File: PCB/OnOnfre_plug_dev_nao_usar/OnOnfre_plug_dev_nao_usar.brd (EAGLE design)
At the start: 44.4 x 47.7 mm, 41 parts, among them IC4 HLW8012, J7 8p, Q3 2N7002, Q4 2N7002, U2 esp12

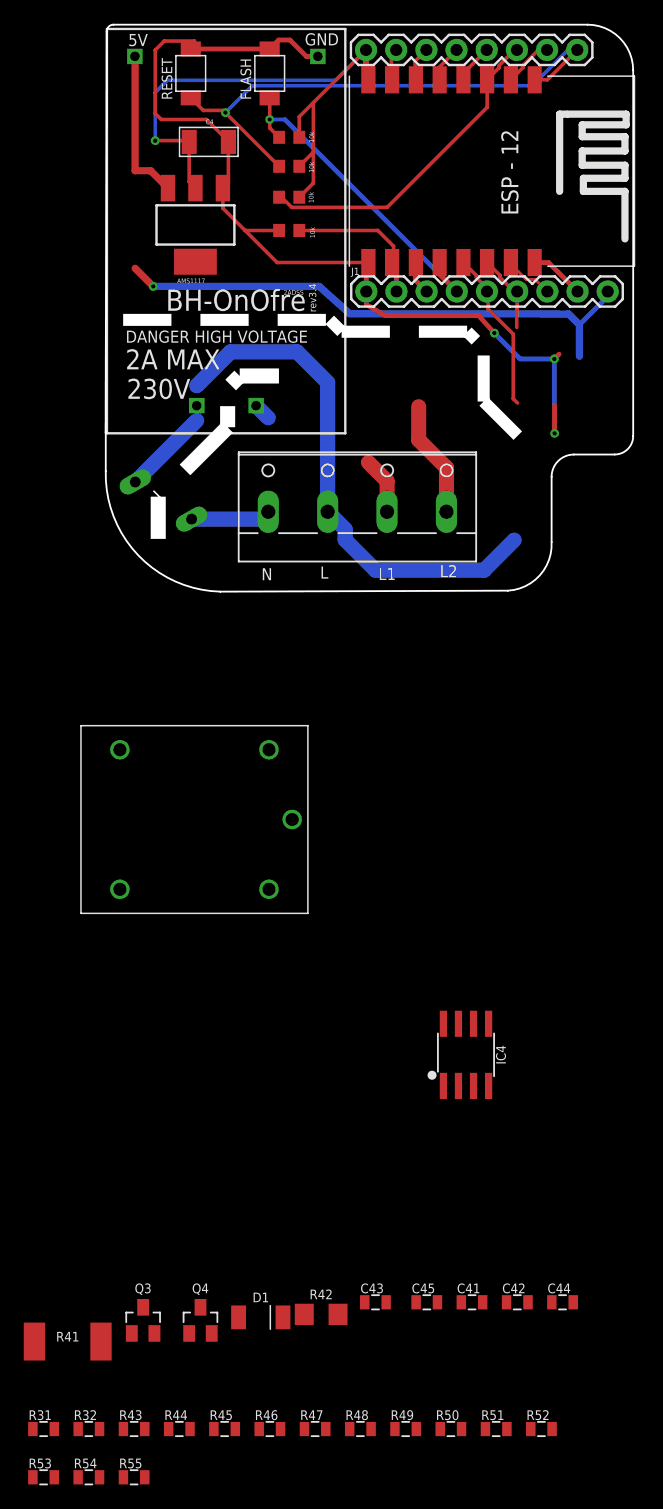
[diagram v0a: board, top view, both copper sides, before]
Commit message: Labels Fix
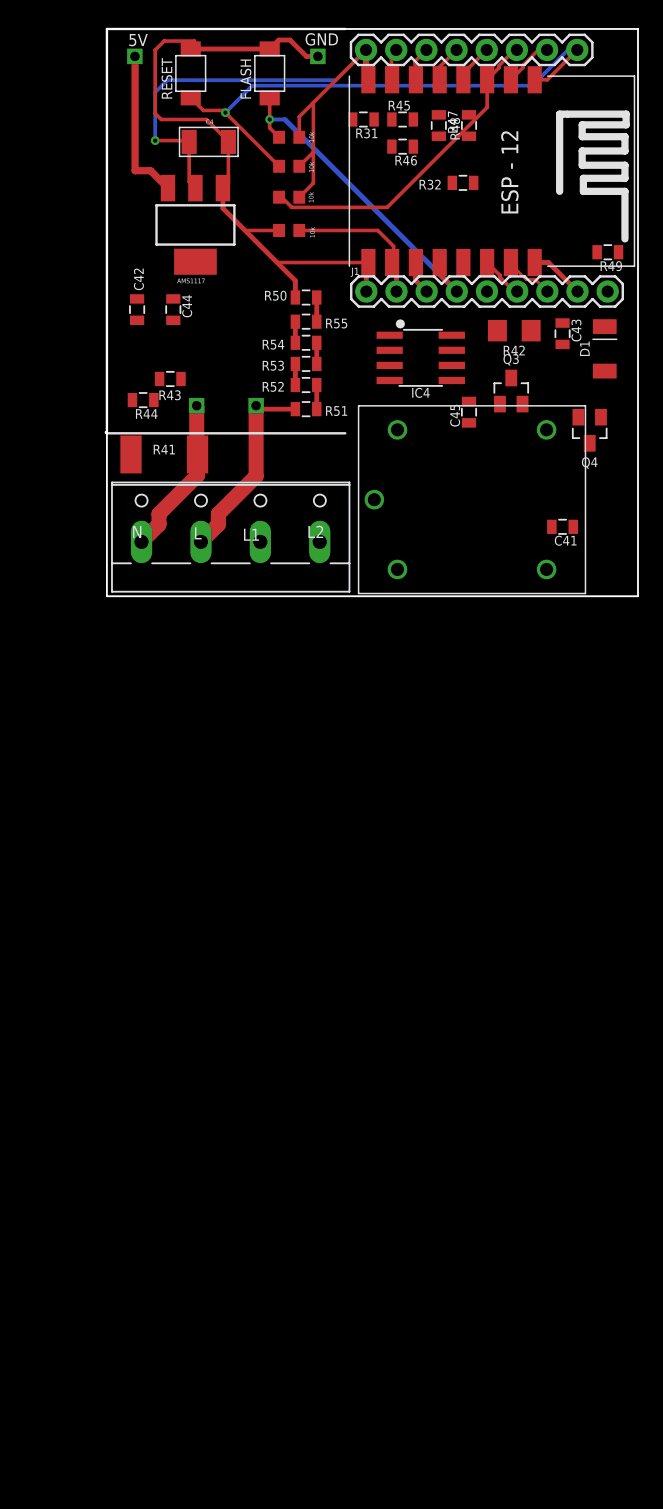
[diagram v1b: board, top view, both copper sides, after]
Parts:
- removed R5: VARISTORS07K230, varistor:S07K230
- moved R31 113.5 mm to (22.1, 38.4), turned to 180 degrees
- moved R45 111.2 mm to (25.4, 38.4)
- moved R47 110.2 mm to (28.4, 37.8), turned to 270 degrees
- moved R48 110.1 mm to (31.0, 37.8), turned to 90 degrees
- moved R32 109.5 mm to (30.5, 33.0), turned to 180 degrees
- moved R46 108.5 mm to (25.4, 36.1), turned to 180 degrees
- moved R49 100.5 mm to (42.7, 27.2), turned to 180 degrees
- moved R55 98.4 mm to (17.3, 21.3), turned to 180 degrees
- moved R54 97.2 mm to (17.3, 19.6), turned to 180 degrees
- moved R53 96.3 mm to (17.3, 17.8), turned to 180 degrees
- moved R50 96.0 mm to (17.3, 23.4)
- moved R52 90.1 mm to (17.3, 16.0), turned to 180 degrees
- moved C44 89.8 mm to (6.10, 22.4), turned to 270 degrees
- moved C42 89.5 mm to (3.05, 22.4), turned to 270 degrees
- moved R43 88.4 mm to (5.84, 16.5)
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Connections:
- net LINE_IN: now also U$2.P$2; no longer R5.1, U$2.P$1
- net NEUTRAL_IN: now also U$2.P$1; no longer R5.2, U$2.P$2
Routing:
- net 5V: track 45.7 -> 0.00 mm, vias 1 -> 0
- net NEUTRAL_IN: track 50.8 -> 17.2 mm
- net GND: track 81.8 -> 63.9 mm, vias 3 -> 0
- net GPIO04: track 13.9 -> 0.00 mm
- net NC: track 9.81 -> 0.00 mm
- net LINE_IN: track 7.28 -> 13.4 mm
- net NO: track 4.80 -> 0.00 mm
- net GPIO05: track 6.68 -> 3.64 mm
- net N$6: track 0.00 -> 2.26 mm
- net V2P: track 0.00 -> 2.03 mm
- net N$8: track 0.00 -> 1.78 mm
- net N$16: track 0.00 -> 1.78 mm
- net N$15: track 0.00 -> 1.78 mm
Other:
- board size 44.4 x 47.7 mm -> 44.8 x 47.8 mm
- board text removed: "230V"
- board text removed: "2A MAX"
- board text removed: "2ADSS"
- board text removed: "BH-OnOfre"
- board text removed: "DANGER HIGH VOLTAGE"
- board text removed: "rev3.4"
